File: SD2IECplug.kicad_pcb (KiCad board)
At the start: 2 copper layers, 50 x 49 mm, 42 parts, among them J1 ISP, J2 X6, J4 IEC, J5 C64-CassettePort, J6 C64-CassettePort, J7 Power, J8 X3, Q1 IRLML2803, Q2 IRLML2803, Q3 IRLML2803, Q4 IRLML2803, U1 ATMEGA644-20AU, U2 LM1117-3.3, Y1 8MHz

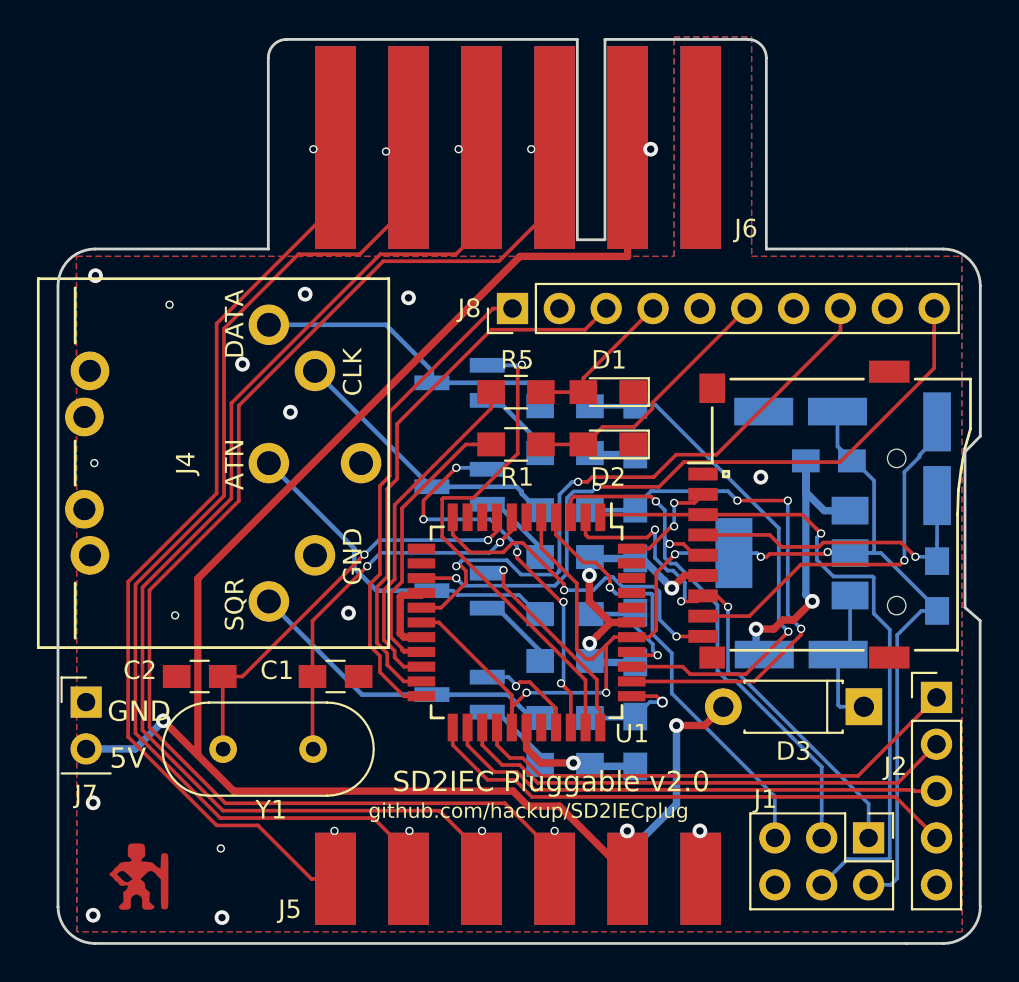
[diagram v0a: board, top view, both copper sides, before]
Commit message: Improved routing.
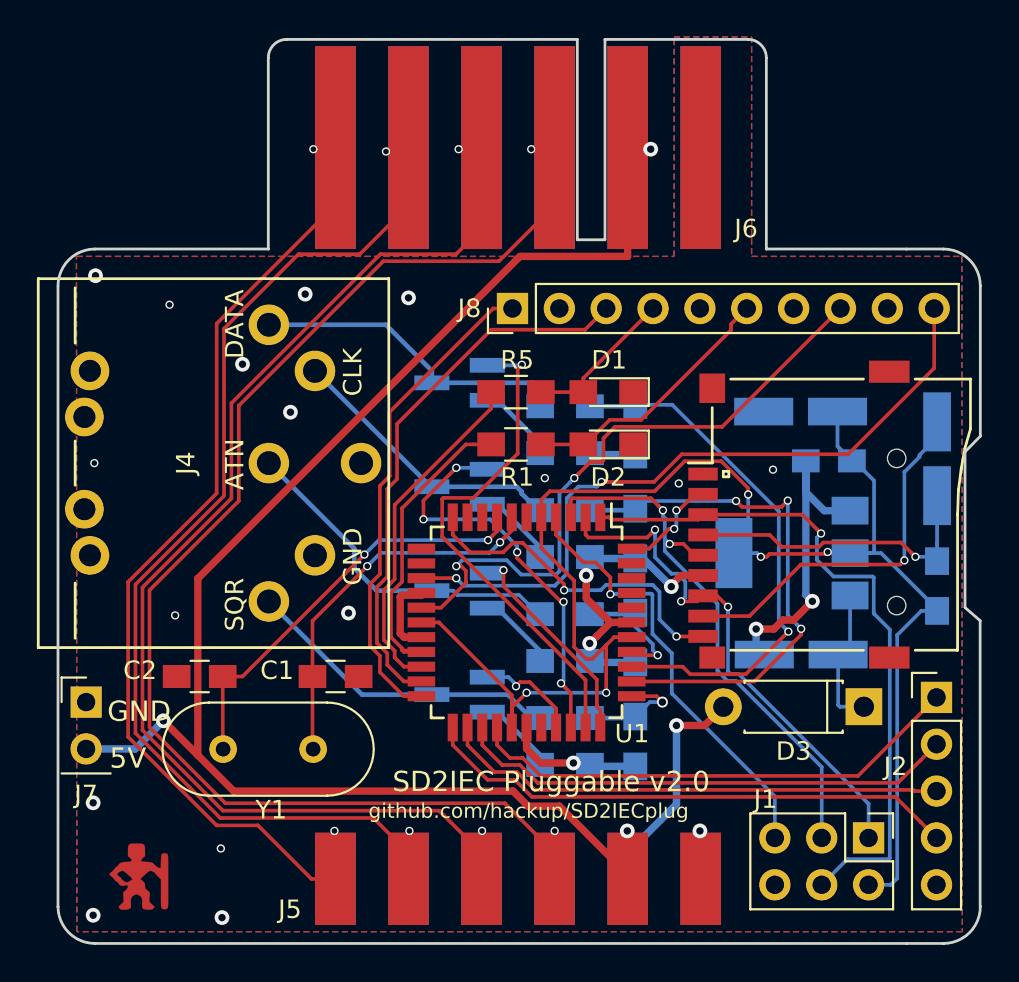
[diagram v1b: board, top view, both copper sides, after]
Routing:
- net +3V3: track 79.4 -> 87.6 mm
- net Net-(R7-Pad2): track 28.5 -> 29.0 mm
- net Cas-GND: track 54.6 -> 55.1 mm, vias 21 -> 23
